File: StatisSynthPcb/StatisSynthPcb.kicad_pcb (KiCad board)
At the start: 2 copper layers, 21 parts, among them J1 Conn_01x02_Pin, J2 PCM5102A, J3 Oled, J4 Conn pin for power amplifier, SW1 SW_Push, SW2 SW_Push, SW3 SW_Push, SW4 SW_Push, SW5 SW_SPST, U3 MCP3208

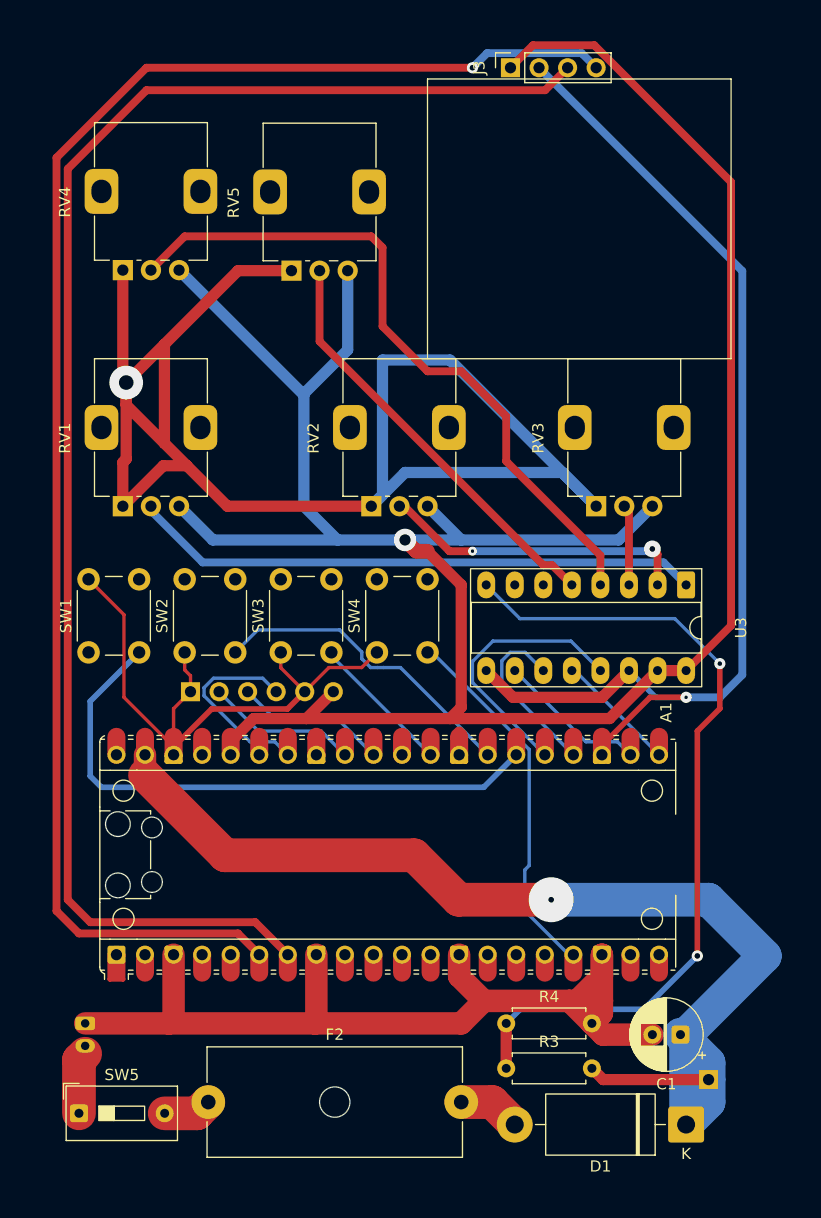
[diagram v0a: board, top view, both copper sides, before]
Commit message: added gerbers photos bom
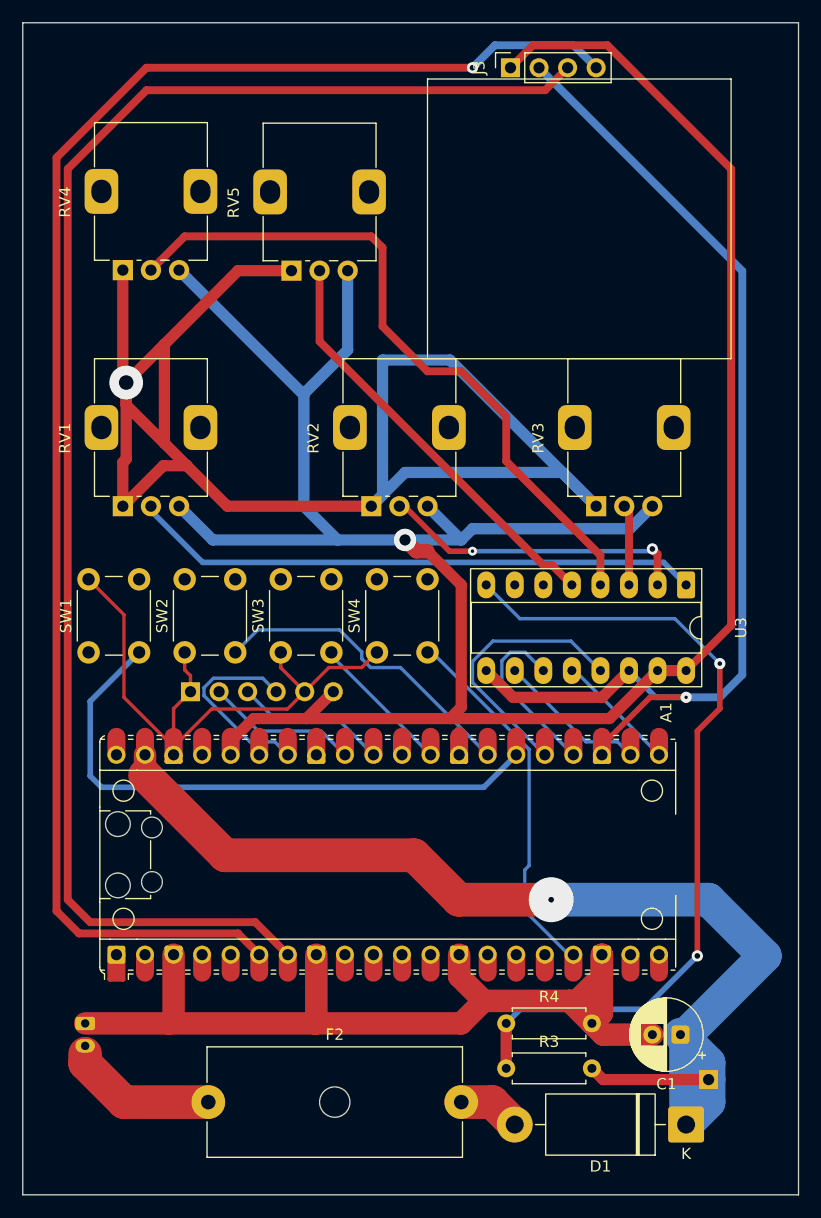
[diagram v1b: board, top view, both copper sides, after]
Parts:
- removed SW5: SW_SPST, Button_Switch_THT:SW_DIP_SPSTx01_Slide_9.78x4.72mm_W7.62mm_P2.54mm
- R4: value 390k -> 330k
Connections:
- F2 pad 1: Net-(SW5-B) -> Net-(J1-Pin_2)
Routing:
- net Net-(J1-Pin_2): track 5.53 -> 14.6 mm
- net Net-(SW5-B): track 4.29 -> 0.00 mm
- net +3.3V: track 228.6 -> 229.3 mm
- net /SDA: track 139.0 -> 139.6 mm
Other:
- board outline added: 69 x 104.2 mm
